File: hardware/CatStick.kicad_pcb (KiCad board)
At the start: 4 copper layers, 80 x 20 mm, 85 parts, among them J1 Antenna, J2 Conn_01x06_Female, J3 JTAG, P1 USB_C_Plug_USB2.0, U1 AP2112K-3.3, U2 RFSW8006QTR7, U3 ATSAMD21E18A, U4 0900PC15A0036, U5 0900FM15D0039, U6 SW409, U7 SX1262IMLTRT, U8 CC1352R1F3RGZR, Y1 48MHz, Y2 32.768kHz, Y3 32Mhz_10pF_10ppm

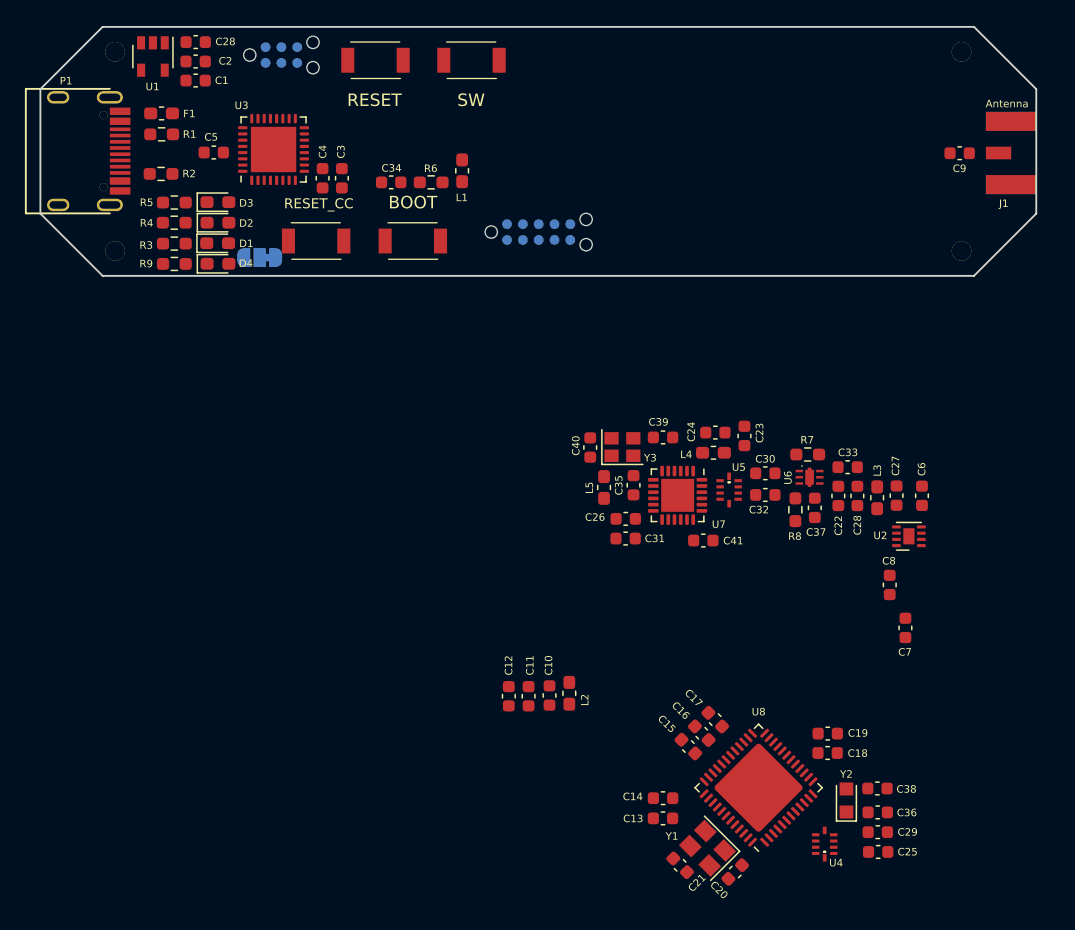
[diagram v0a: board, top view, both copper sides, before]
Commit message: NewFloorPlan
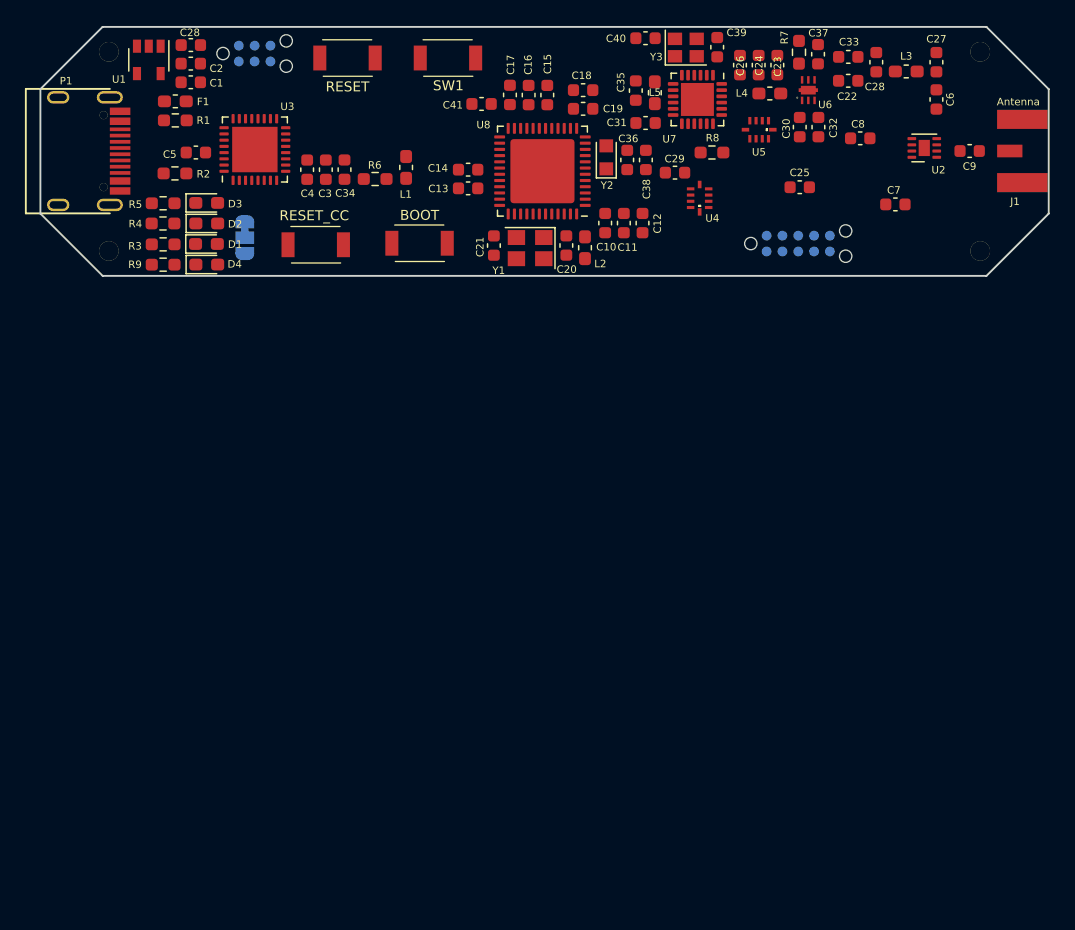
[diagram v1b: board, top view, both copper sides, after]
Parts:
- moved C18 56.8 mm to (128.6, 105.1)
- moved C36 56.1 mm to (132.1, 110.7), turned to 90 degrees
- moved C29 55.4 mm to (136.0, 111.7), turned to 0 degrees
- moved Y2 55.1 mm to (130.5, 110.5)
- moved C19 53.9 mm to (128.6, 106.6)
- moved C38 53.8 mm to (133.6, 110.7), turned to 270 degrees
- moved C25 53.8 mm to (146.0, 112.9)
- moved C15 53.5 mm to (125.7, 105.5), turned to 90 degrees
- moved C16 53.1 mm to (124.2, 105.5), turned to 90 degrees
- moved C13 53.0 mm to (119.4, 113.0)
- moved C14 52.9 mm to (119.4, 111.5)
- moved U4 52.9 mm to (138.0, 112.8)
- moved C17 52.8 mm to (122.7, 105.5), turned to 90 degrees
- moved U8 52.5 mm to (125.3, 111.6), turned to 180 degrees
- moved C20 52.1 mm to (127.2, 117.6), turned to 270 degrees
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- renumbered SW to SW1
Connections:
- net /RF_N_2_4_GHZ renamed /2_4_GHZ_RF_N
- net /RF_N_SUB_1_GHZ renamed /SUB_1_GHZ_RF_N
- net /RF_P_2_4_GHZ renamed /2_4_GHZ_RF_P
- net /RF_P_SUB_1_GHZ renamed /SUB_1_GHZ_RF_P
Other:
- board size 80 x 20 mm -> 81 x 20 mm
